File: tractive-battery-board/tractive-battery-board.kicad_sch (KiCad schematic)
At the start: 96 parts, among them J1 FTSH-107-01-F-DV-K-P-TR, J2 IMD_Connector, J3 Busbar_Temp_Sense, J4 Cooling_TS, J5 E-Meter, J6 BMS_TS, J7 Conn_02x13_Counter_Clockwise, Q1 AO3400A, Q2 AO3401A, SW1 Y97KT23B5NAFP, SW2 SW_Push, U1 STLINK-V3MODS, U2 STM32G473RBT6, U3 ISO1044BD, U4 ISO1044BD, U5 DS18B20Z+, U6 MIC5504-3.3YM5, U7 AP63205WU, Y1 ECS-240-8-37B-CKY-TR

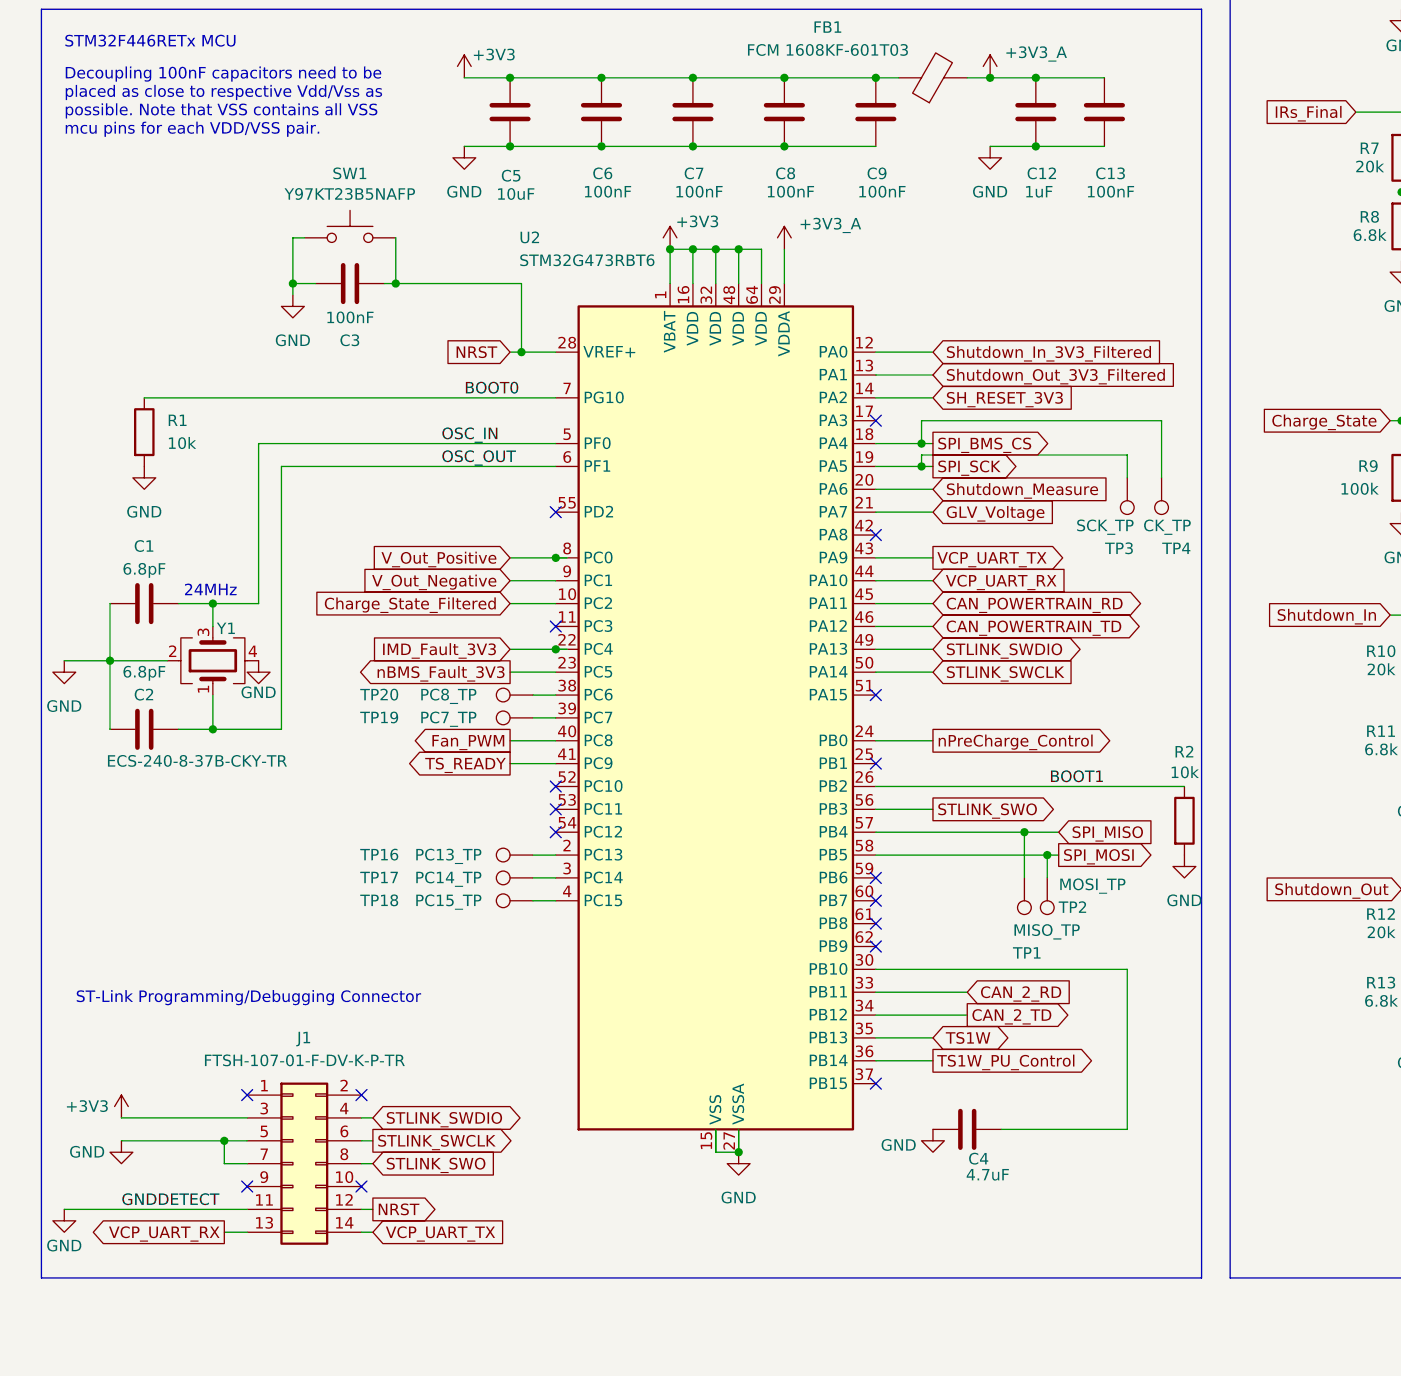
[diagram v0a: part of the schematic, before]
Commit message: Fixed MCU PINs
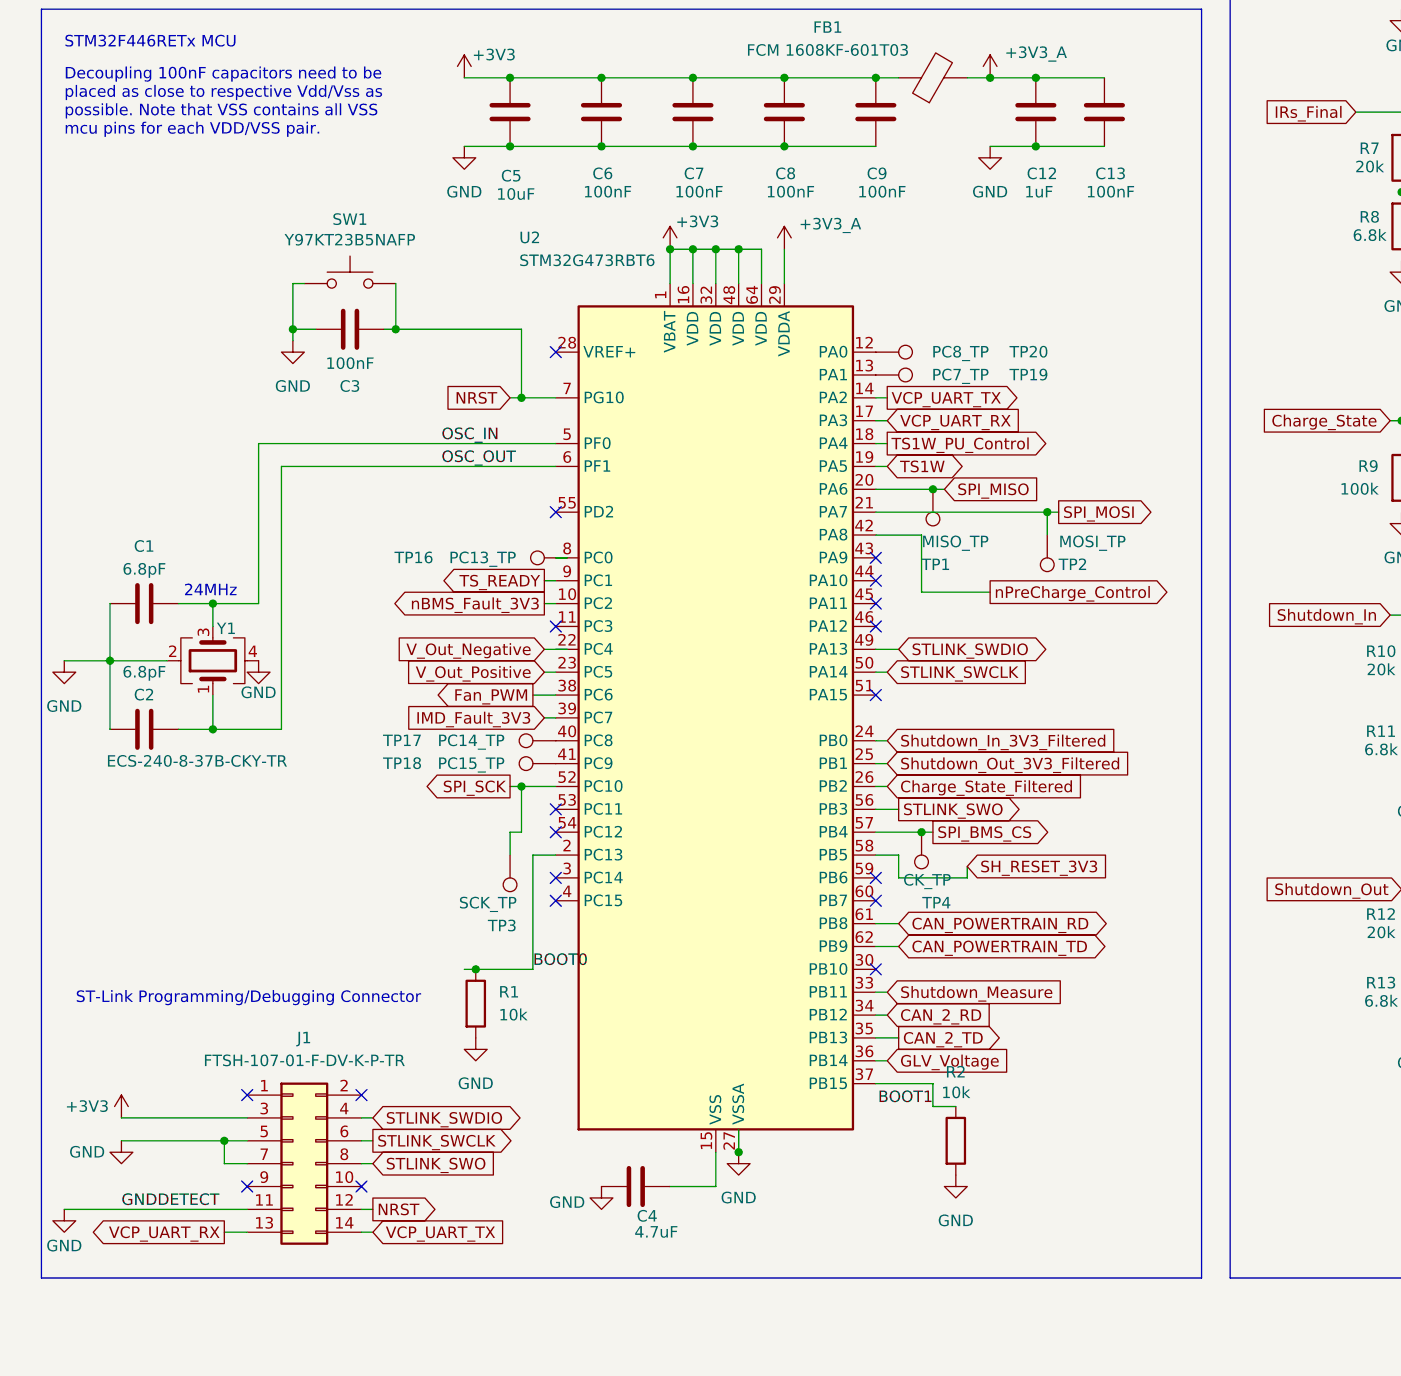
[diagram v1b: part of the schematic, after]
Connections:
- net BOOT0: now also U2.2 (PC13); no longer U2.7 (PG10)
- net BOOT1: now also U2.37 (PB15); no longer U2.26 (PB2)
- net CAN_2_RD: now also U2.34 (PB12); no longer U2.33 (PB11)
- net CAN_2_TD: now also U2.35 (PB13); no longer U2.34 (PB12)
- net CAN_POWERTRAIN_RD: now also U2.61 (PB8); no longer U2.45 (PA11)
- net CAN_POWERTRAIN_TD: now also U2.62 (PB9); no longer U2.46 (PA12)
- net Charge_State_Filtered: now also U2.26 (PB2); no longer U2.10 (PC2)
- net Fan_PWM: now also U2.38 (PC6); no longer U2.40 (PC8)
- net GLV_Voltage: now also U2.36 (PB14); no longer U2.21 (PA7)
- net GND: no longer U2.15 (VSS), U2.31 (VSS), U2.47 (VSS), U2.63 (VSS)
- net IMD_Fault_3V3: now also U2.39 (PC7); no longer U2.22 (PC4)
- net NRST: now also U2.7 (PG10); no longer U2.28 (VREF+)
- net SH_RESET_3V3: now also U2.58 (PB5); no longer U2.14 (PA2)
- net SPI_BMS_CS: now also U2.57 (PB4); no longer U2.18 (PA4)
- net SPI_MISO: now also U2.20 (PA6); no longer U2.57 (PB4)
- net SPI_MOSI: now also U2.21 (PA7); no longer U2.58 (PB5)
- net SPI_SCK: now also U2.52 (PC10); no longer U2.19 (PA5)
- net Shutdown_In_3V3_Filtered: now also U2.24 (PB0); no longer U2.12 (PA0)
- net Shutdown_Measure: now also U2.33 (PB11); no longer U2.20 (PA6)
- net Shutdown_Out_3V3_Filtered: now also U2.25 (PB1); no longer U2.13 (PA1)
- net TS1W: now also U2.19 (PA5); no longer U2.35 (PB13)
- net TS1W_PU_Control: now also U2.18 (PA4); no longer U2.36 (PB14)
- net TS_READY: now also U2.9 (PC1); no longer U2.41 (PC9)
- net VCP_UART_RX: now also U2.17 (PA3); no longer U2.44 (PA10)
- net VCP_UART_TX: now also U2.14 (PA2); no longer U2.43 (PA9)
- net V_Out_Negative: no longer U2.9 (PC1)
- net V_Out_Positive: now also U2.23 (PC5); no longer U2.8 (PC0)
- net nBMS_Fault_3V3: now also U2.10 (PC2); no longer U2.23 (PC5)
- net nPreCharge_Control: now also U2.42 (PA8); no longer U2.24 (PB0)
- net at TP16.1: now also U2.8 (PC0); no longer U2.2 (PC13)
- net at U2.3 (PC14): no longer TP17.1
- net at C4.2: now also U2.15 (VSS), U2.31 (VSS), U2.47 (VSS), U2.63 (VSS); no longer U2.30 (PB10)
- net at TP20.1: now also U2.12 (PA0); no longer U2.38 (PC6)
- net at TP19.1: now also U2.13 (PA1); no longer U2.39 (PC7)
- net at U2.4 (PC15): no longer TP18.1
- new net: TP17.1, U2.40 (PC8)
- new net: TP18.1, U2.41 (PC9)
- no-connect marks 36 -> 37
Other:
- moved on the sheet: C3, C4, R1, R2, SW1, TP1, TP16, TP17, TP18, TP19, TP2, TP20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
